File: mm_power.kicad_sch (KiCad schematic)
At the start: 1 part, among them J5 Conn_01x02

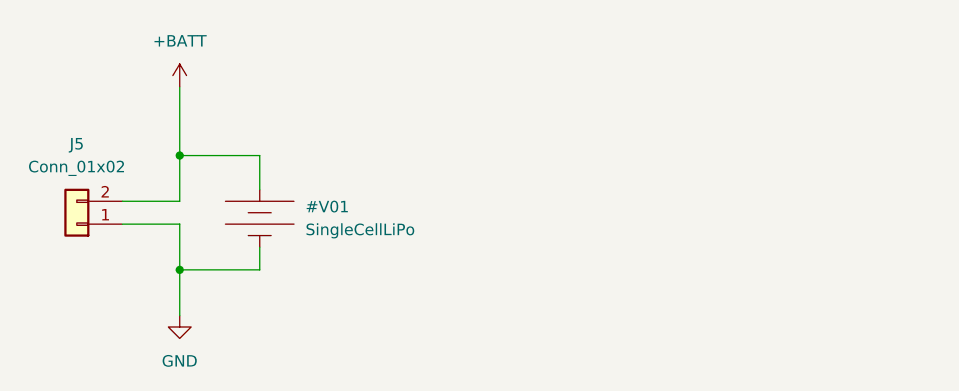
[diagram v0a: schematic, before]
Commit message: fin tp2
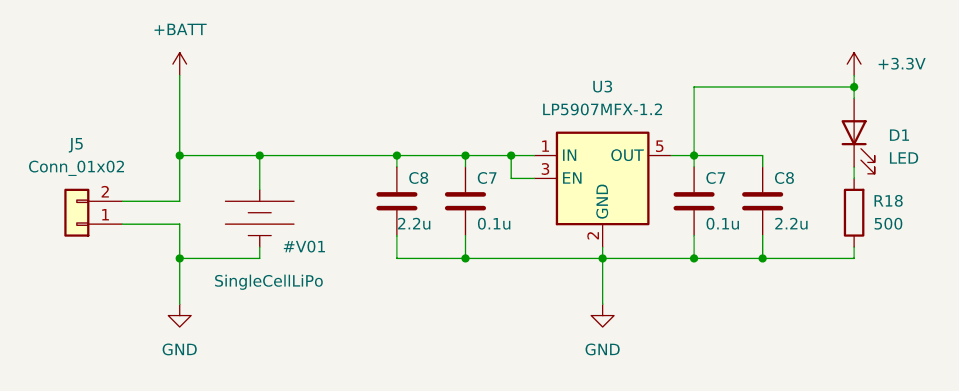
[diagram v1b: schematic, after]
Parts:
- added C7 (x2): 0.1u, Capacitor_SMD:C_0603_1608Metric, symbol Device:C
- added C8 (x2): 2.2u, Capacitor_SMD:C_0603_1608Metric, symbol Device:C
- added D1: LED, LED_SMD:LED_0603_1608Metric, symbol Device:LED
- added R18: 500, Resistor_SMD:R_0603_1608Metric, symbol Device:R
- added U3: LP5907MFX-1.2, Package_TO_SOT_SMD:SOT-23-5, symbol Regulator_Linear:LP5907MFX-1.2
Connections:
- net +BATT: now also C7.1, C8.1, U3.1 (IN), U3.3 (EN)
- net GND: now also C7.2, C7.2, C8.2, C8.2, R18.1, U3.2 (GND)
- new net: D1.1 (K), R18.2
- new net +3.3V: C7.1, C8.1, D1.2 (A), U3.5 (OUT)
